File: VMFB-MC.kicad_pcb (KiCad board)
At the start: 2 copper layers, 64.6 x 77 mm, 53 parts, among them J1 DISPENSE, J10 PIR, J2 EMPTY, J3 DISPENSE, J4 DEPOSIT, J5 Conn_01x03_Pin, J6 DISPENSE, J7 EMPTY, J8 MOTOR, J9 Conn_01x10_Pin, Q1 Q_Photo_NPN, Q10 Q_Photo_NPN, Q2 Q_Photo_NPN, Q3 Q_Photo_NPN, Q4 Q_Photo_NPN, Q5 Q_Photo_NPN, Q6 Q_Photo_NPN, Q7 TIP120, Q8 TIP120, Q9 BC337, U1 LM393

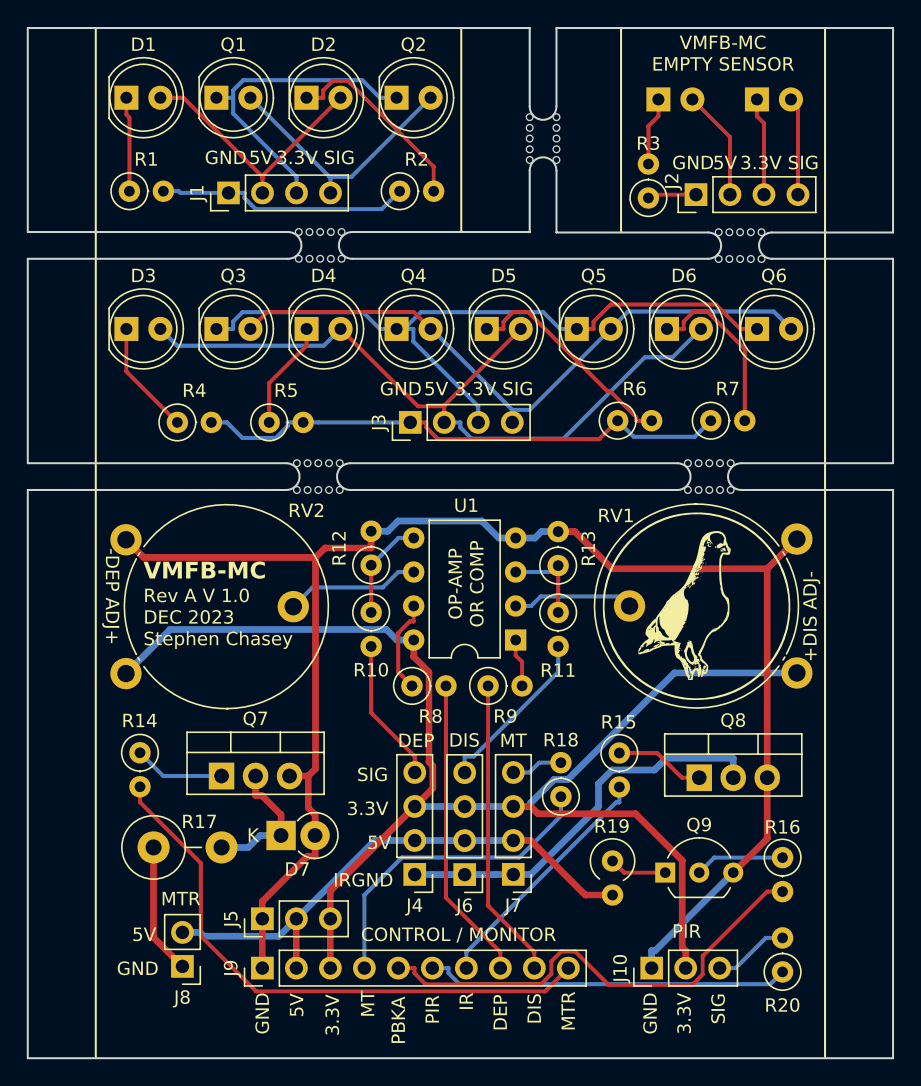
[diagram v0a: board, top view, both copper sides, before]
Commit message: Layout tweaks
more layout and labelling tweaks
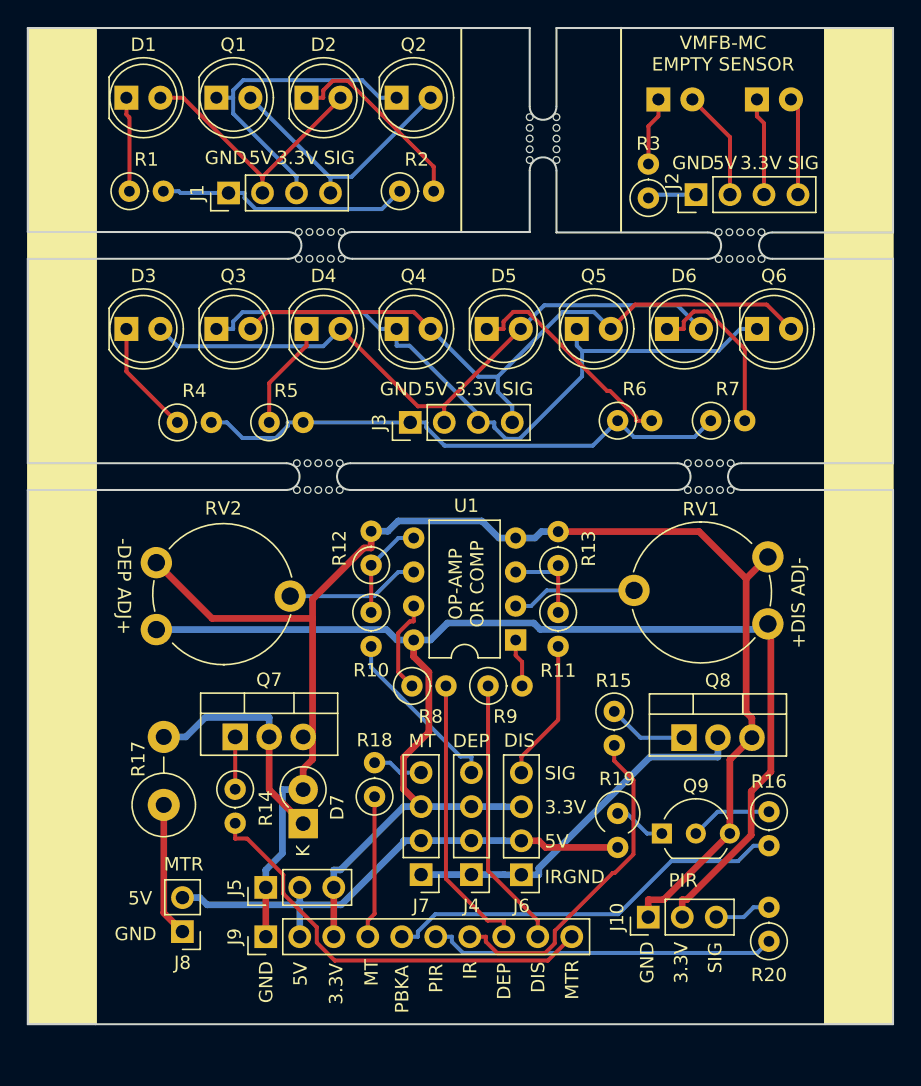
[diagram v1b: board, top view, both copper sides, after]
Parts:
- removed LOGO_BACK, LOGO_FRONT: LOGO, VMFB:VMFB_logo_14mm
- added G***: LOGO, VMFB-MC:VMFB_logo_20mm, B.Cu at (132.8, 97.3)
- RV1, RV2: footprint Potentiometer_THT:Potentiometer_Piher_PT-15-V02_Vertical -> Potentiometer_THT:Potentiometer_Piher_PT-10-V10_Vertical
- moved R18 13.9 mm to (126.0, 107.5)
- moved R14 7.62 mm to (115.6, 106.9)
- moved J7 6.89 mm to (129.5, 113.3)
- moved J4 4.24 mm to (133.2, 113.3)
- moved J6 4.24 mm to (137.0, 113.3)
- moved RV2 3.99 mm to (109.7, 95.0)
- moved J10 3.82 mm to (146.4, 116.5)
- moved R16 3.58 mm to (155.4, 108.6)
- moved R19 3.58 mm to (144.1, 108.7)
- moved R17 3.27 mm to (110.2, 108.1), turned to 90 degrees
- moved Q8 3.20 mm to (149.1, 103.1)
- moved R15 3.13 mm to (143.9, 101.1)
- moved Q7 3.09 mm to (115.6, 103.0)
- moved Q9 2.93 mm to (147.4, 110.2)
- moved J8 2.60 mm to (111.6, 117.5)
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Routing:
- net EMPTY: track 24.0 -> 10.7 mm
- net GND: track 123.4 -> 111.0 mm
- net MOTOR: track 42.9 -> 32.3 mm
- net Net-(D3-A): track 57.3 -> 49.0 mm
- net MOTOR GND RES: track 10.3 -> 17.5 mm
- net SENSOR IR: track 18.4 -> 25.3 mm
- net PBKA: track 35.7 -> 30.5 mm
- net Net-(Q7-B): track 6.82 -> 3.91 mm
- net Net-(J3-Pin_4): track 48.5 -> 50.8 mm
- net IR GND: track 29.9 -> 27.6 mm
- net DEPOSIT SIG: track 10.8 -> 13.0 mm
- net DISPENSE: track 22.5 -> 20.3 mm
- net DISPENSE SIG: track 12.7 -> 10.6 mm
- net +5V: track 40.6 -> 38.7 mm
- net DEPOSIT: track 22.8 -> 21.2 mm
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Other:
- board size 64.6 x 77 mm -> 64.6 x 74.4 mm
- board text added: "VMFB-MC Rev A V 1.0 DEC 2023 Stephen Chasey"
- board text removed: "CONTROL / MONITOR"
- board text removed: "Rev A V 1.0 DEC 2023 Stephen Chasey"
- board text removed: "VMFB-MC"
